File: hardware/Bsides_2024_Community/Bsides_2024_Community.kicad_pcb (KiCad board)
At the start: 2 copper layers, 169.6 x 159.5 mm, 42 parts, among them J1 Conn_02x03_Odd_Even, J2 Battery, J3 Battery, J4 OLED, J5 Conn_01x05, J6 Conn_01x05, P1 USB_C_Plug_USB2.0, Q1 DMG3415U-7, SW1 ON, SW2 RESET, SW3 BOOT, SW4 RESET, SW6 RESET, U1 ESP32-C6-WROOM-1U-N4, U2 AP2112K-3.3

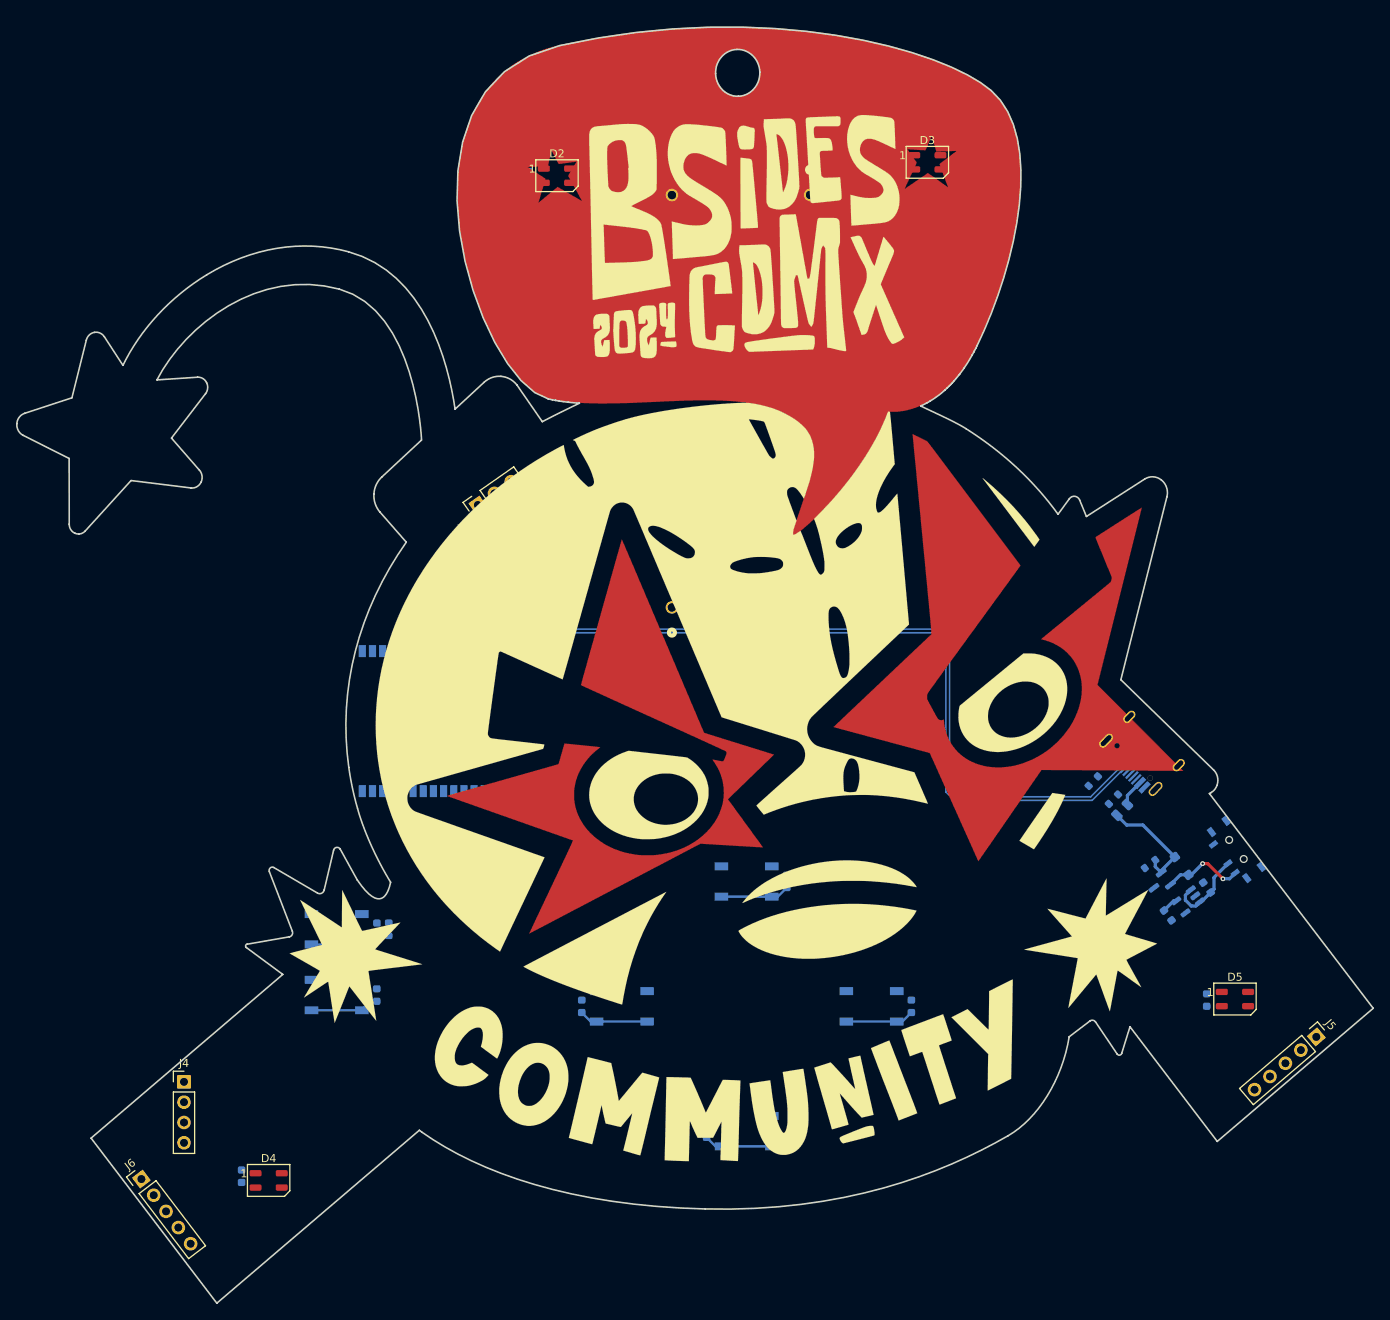
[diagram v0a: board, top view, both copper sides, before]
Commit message: feat(Hw): Update PCB
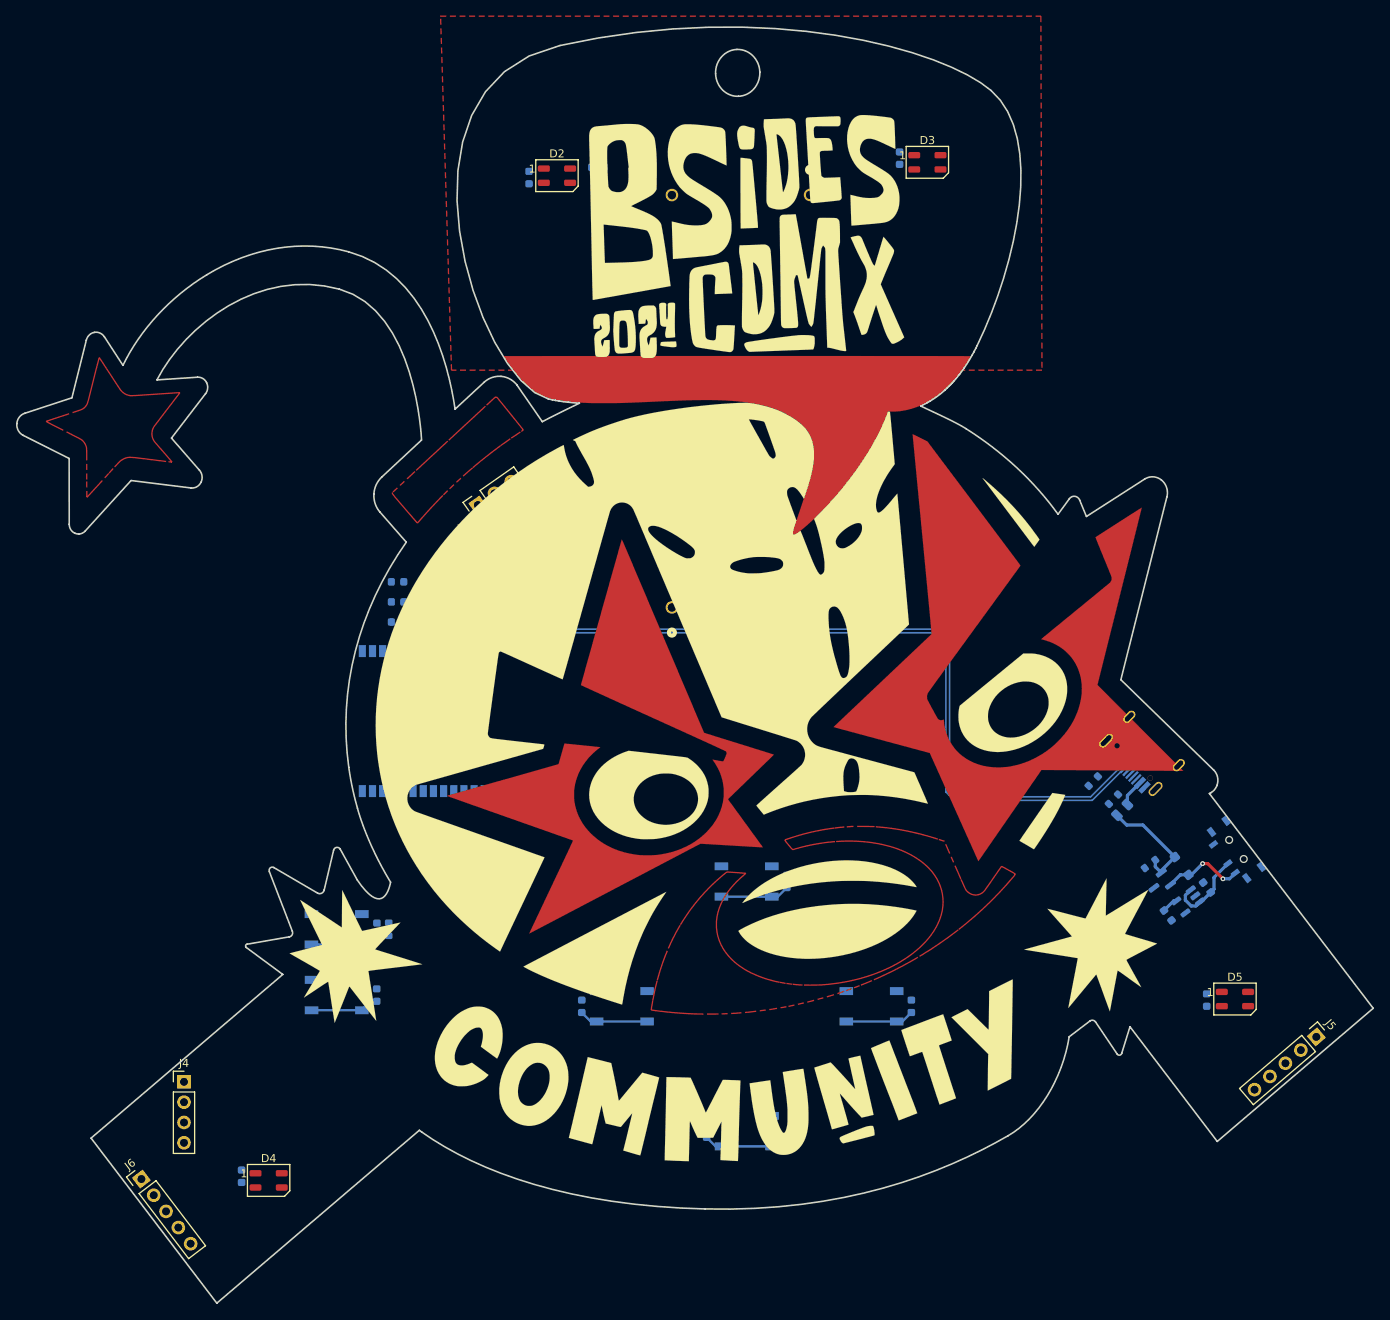
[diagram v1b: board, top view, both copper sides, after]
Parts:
- added C13: 1uF, Capacitor_SMD:C_0603_1608Metric, B.Cu at (99.0, 90.5)
- added C14: 10uF, Capacitor_SMD:C_0603_1608Metric, B.Cu at (99.0, 93.0)
- added C15: 10uF, Capacitor_SMD:C_0603_1608Metric, B.Cu at (99.0, 95.5)
- J1: value Conn_02x03_Odd_Even -> Add_On
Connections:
- C1 pad 1: Net-(SW1-B) -> VBUS
- C12 pad 2: +3V3 -> /VOUT
- C2 pad 1: +3V3 -> Net-(D1-A)
- C5 pad 2: +3V3 -> /VOUT
- C6 pad 2: +3V3 -> /VOUT
- C7 pad 2: +3V3 -> /VOUT
- D1 pad 2: VBUS -> Net-(D1-A)
- D2 pad 1: +3V3 -> /VOUT
- D3 pad 1: +3V3 -> /VOUT
- D4 pad 1: +3V3 -> /VOUT
- D5 pad 1: +3V3 -> /VOUT
- J1 pad 1: unconnected-(J1-Pin_1-Pad1) -> /VOUT
- J1 pad 2: unconnected-(J1-Pin_2-Pad2) -> GND
- J1 pad 3: unconnected-(J1-Pin_3-Pad3) -> /SDA
- J1 pad 4: unconnected-(J1-Pin_4-Pad4) -> /SCL
- J4 pad 1: +3V3 -> /VOUT
- Q1 pad 1: VBUS -> Net-(D1-A)
- R1 pad 2: +3V3 -> /VOUT
- R2 pad 1: VBUS -> Net-(D1-A)
- R5 pad 2: +3V3 -> /VOUT
- SW1 pad 2: Net-(SW1-B) -> /VOUT
- U1 pad 2: +3V3 -> /VOUT
- U2 pad 1: Net-(SW1-B) -> VBUS
- U2 pad 3: Net-(SW1-B) -> VBUS
- U2 pad 5: +3V3 -> Net-(D1-A)
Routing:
- net VBUS: track 14.0 -> 24.2 mm
- net Net-(SW1-B): track 10.3 -> 0.00 mm
- net Net-(D1-A): track 0.00 -> 2.04 mm
- net +3V3: track 2.04 -> 0.00 mm
- added copper zone on F.Cu, net (none)
- added copper zone on F.Cu, net GND
